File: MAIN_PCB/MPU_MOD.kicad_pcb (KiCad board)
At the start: 8 copper layers, 50 x 70 mm, 301 parts, among them J1001 FH12-30S-0.5SH_55_, J1101 USB4510-03-1-A_REVA, J1102 USB4510-03-1-A_REVA, J501 MEM2090-00-145-00-A_REVA, J601 M40-3100645R, J701 FTSH-107-01-L-DV-K-A, Q1001 DMG1012TQ-7, Q1002 DMG1012TQ-7, Q1003 DMG1012TQ-7, Q201 DMG1013T-7, U1001 TPS61042DRBR, U1101 HSP051-4M10, U1102 HSP051-4M10, U201 TPS62840DLCR, U202 STPMIC1APQR, U301 STM32MP157FABx, U401 MT41K256M16TW-107_P, U501 HSP051-4M10, U502 HSP051-4M10, U601 HSP051-4M10, U602 HSP051-4M10, U701 HSP051-4M10, U702 HSP051-4M10, U901 MAYA-W166-00B, U902 SIT1533AI-H4-DCC-32.768E, Y601 NX2012SA-32.768K, Y701 ECS-2520MVQ-240

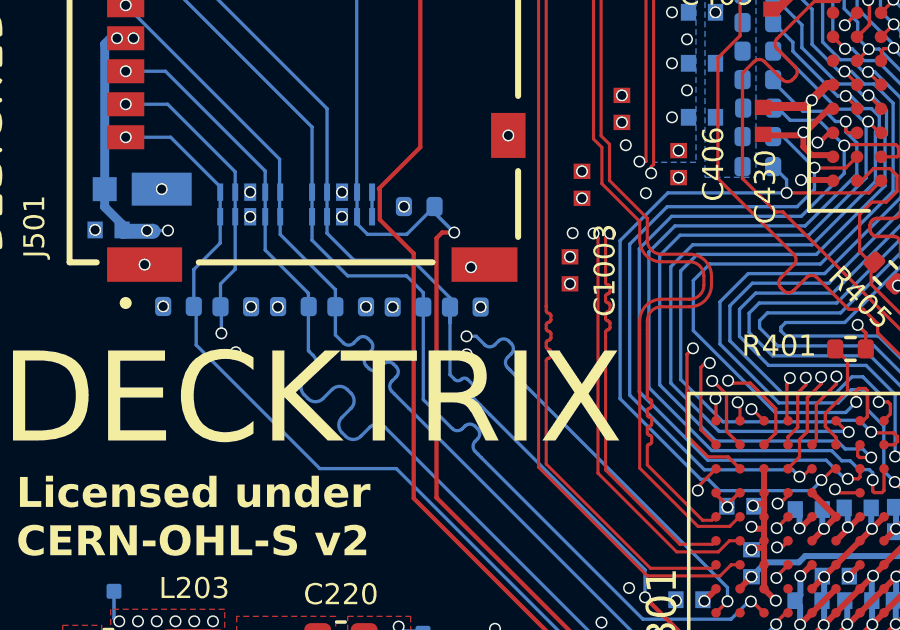
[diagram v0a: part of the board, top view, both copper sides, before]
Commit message: Ready to order
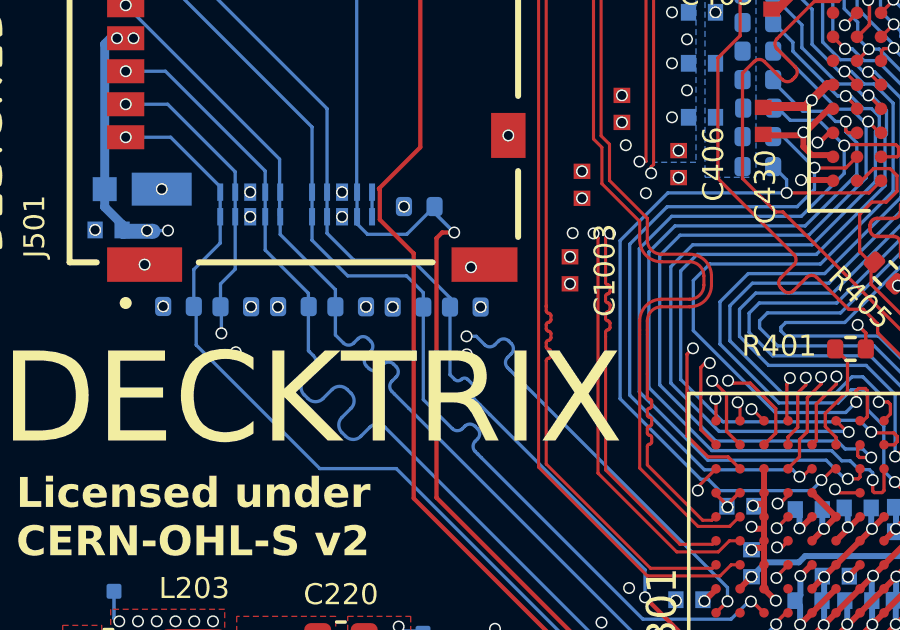
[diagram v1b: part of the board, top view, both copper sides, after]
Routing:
- net SDMMC1_D1: track 35.1 -> 34.6 mm
